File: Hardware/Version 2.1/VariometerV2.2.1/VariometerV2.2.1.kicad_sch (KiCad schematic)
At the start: 21 parts, among them IC1 ESP32-S3-WROOM, SW1 Switch_SW_Push, SW2 Switch_SW_Push

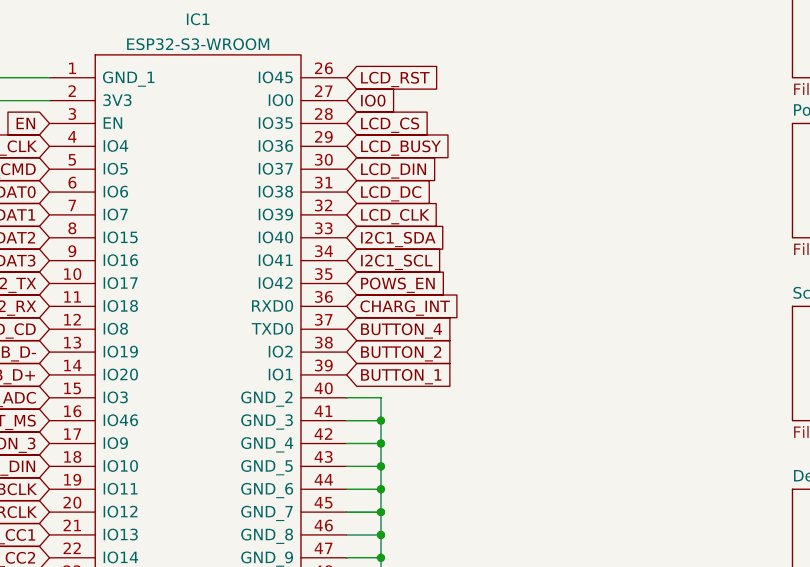
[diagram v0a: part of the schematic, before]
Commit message: Start on pcb
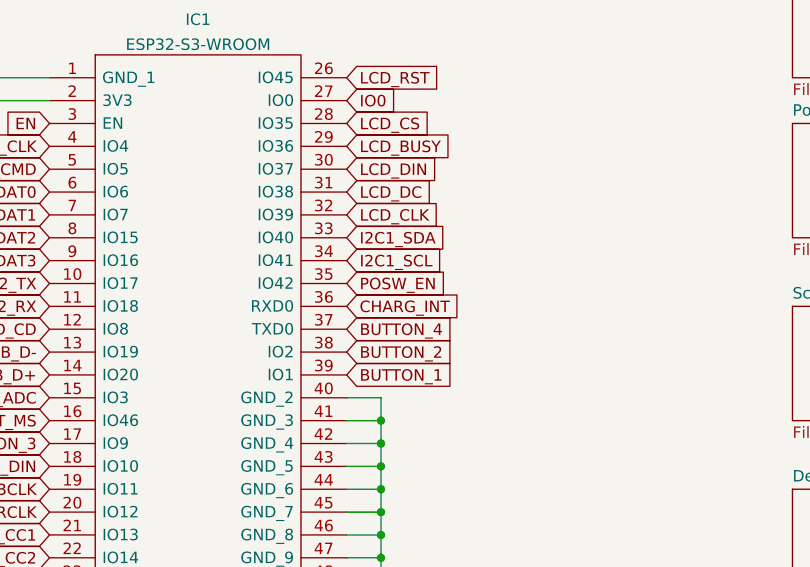
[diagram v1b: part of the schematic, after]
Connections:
- net POWS_EN renamed POSW_EN
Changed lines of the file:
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@@
     )
   )
-  (global_label "POWS_EN" (shape input) (at 154.94 73.66 0) (fields_autoplaced)
+  (global_label "POSW_EN" (shape input) (at 154.94 73.66 0) (fields_autoplaced)
     (effects (font (size 1.27 1.27)) (justify left))
     (property "Intersheetrefs" "${INTERSHEET_REFS}" (at 166.5543 73.66 0)
